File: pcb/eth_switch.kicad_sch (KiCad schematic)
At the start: 110 parts, among them IC1 IP175G, J3 100616-2, J4 Conn_01x04, J5 Conn_01x02, T1 H1102NL, U3 24LC02, U4 USBLC6-2SC6, U5 USBLC6-2SC6, Y2 3225-25M-SR

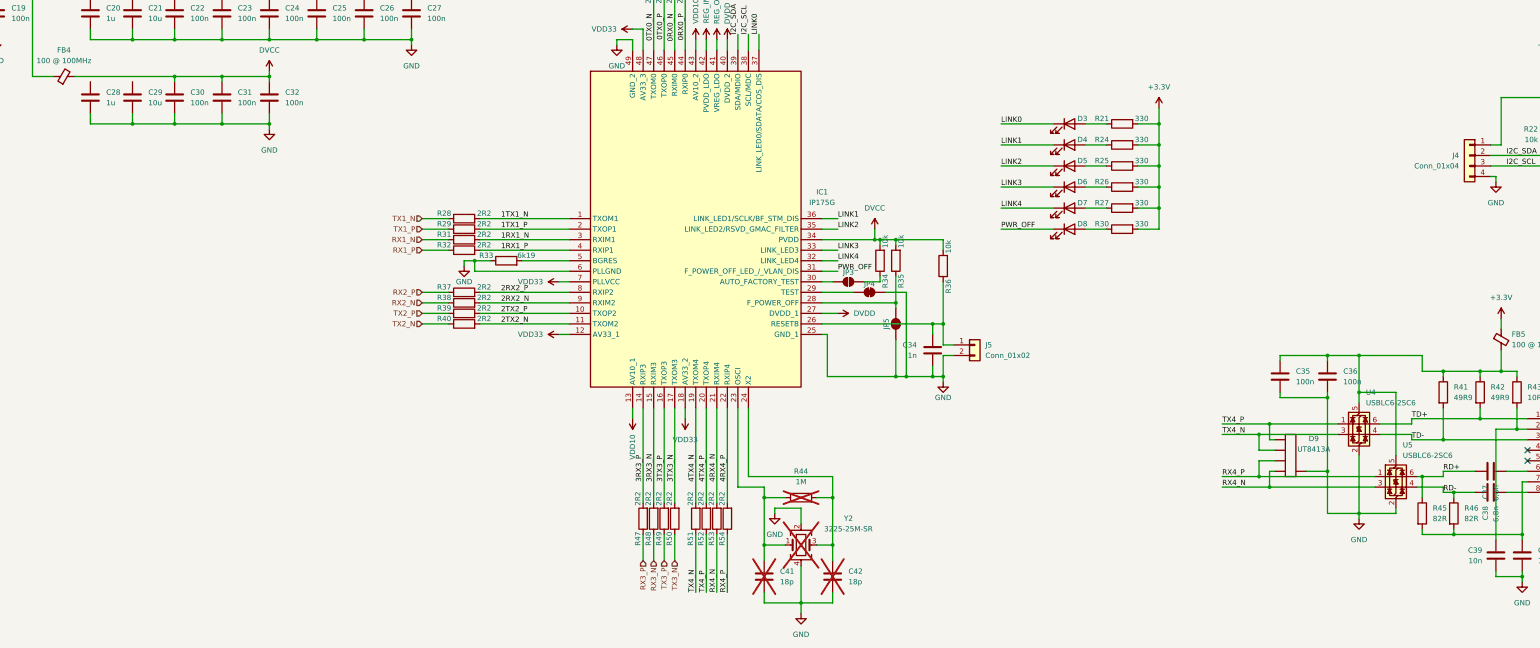
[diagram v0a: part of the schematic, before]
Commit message: Routing
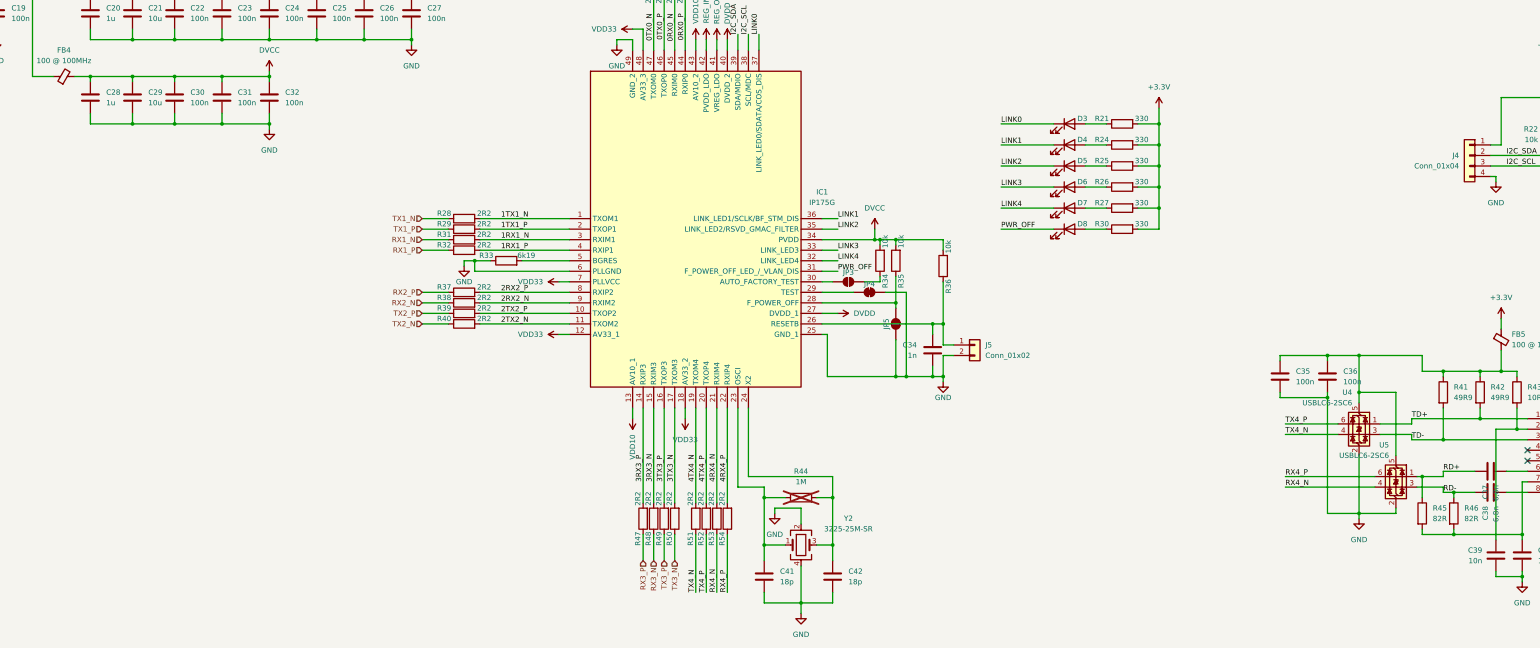
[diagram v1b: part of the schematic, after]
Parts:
- removed D9: UT8413A, Package_DFN_QFN:Diodes_UDFN-10_1.0x2.5mm_P0.5mm, symbol Conn:UT8413A
- C41, C42, Y2: now fitted
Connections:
- net DVCC: now also C28.1, C29.1
- net RD+: now also U5.1 (I/O1); no longer U5.6 (I/O1)
- net RD-: now also U5.3 (I/O2); no longer U5.4 (I/O2)
- net RX4_N: now also U5.4 (I/O2); no longer U5.3 (I/O2)
- net RX4_P: now also U5.6 (I/O1); no longer U5.1 (I/O1)
- net TD+: now also U4.1 (I/O1); no longer U4.6 (I/O1)
- net TD-: now also U4.3 (I/O2); no longer U4.4 (I/O2)
- net TX4_N: now also U4.4 (I/O2); no longer U4.3 (I/O2)
- net TX4_P: now also U4.6 (I/O1); no longer U4.1 (I/O1)
